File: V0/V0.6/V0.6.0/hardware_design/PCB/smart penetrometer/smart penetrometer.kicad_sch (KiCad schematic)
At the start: 33 parts, among them J1 Screw_Terminal, J2 Conn_01x02, J3 Conn_01x02, J4 Conn_01x07_Female, J5 Conn_02x04, U1 VO615A, U2 ADP7157-3.3, U3 ADS1118IDGS, U4 DS3231M, U5 BME260

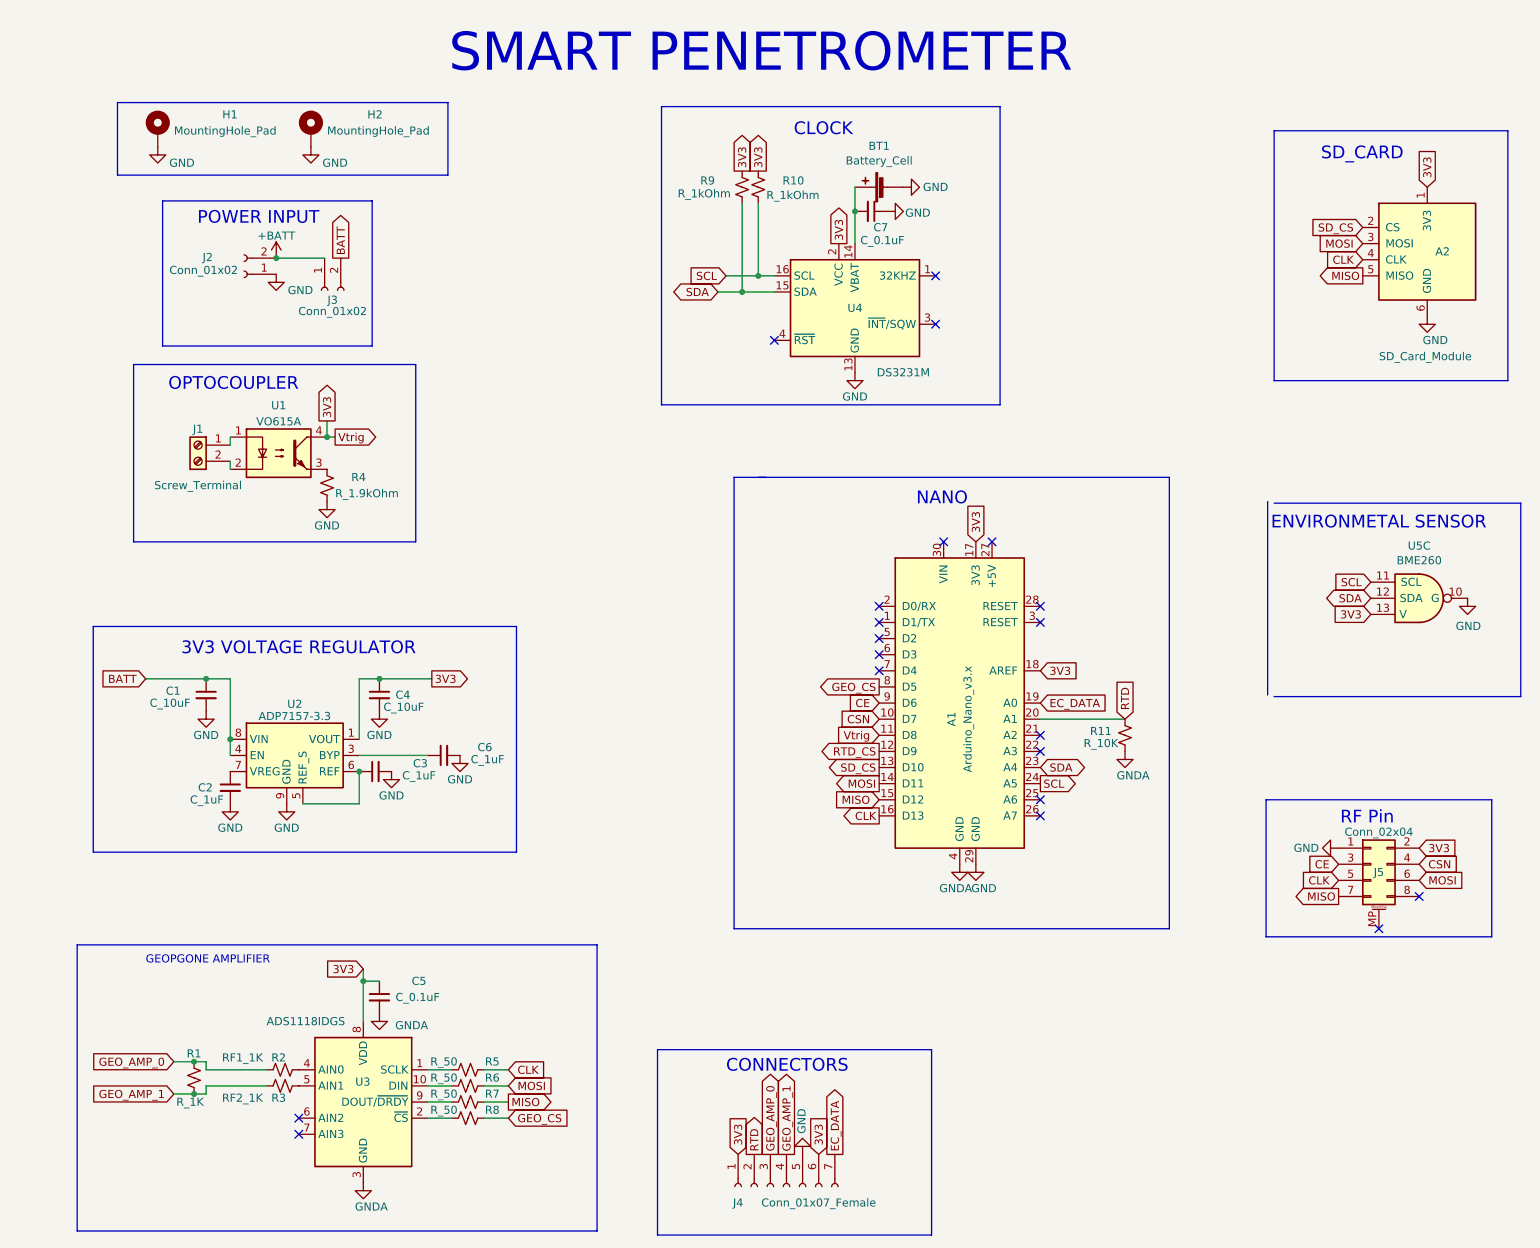
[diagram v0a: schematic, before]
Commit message: correction
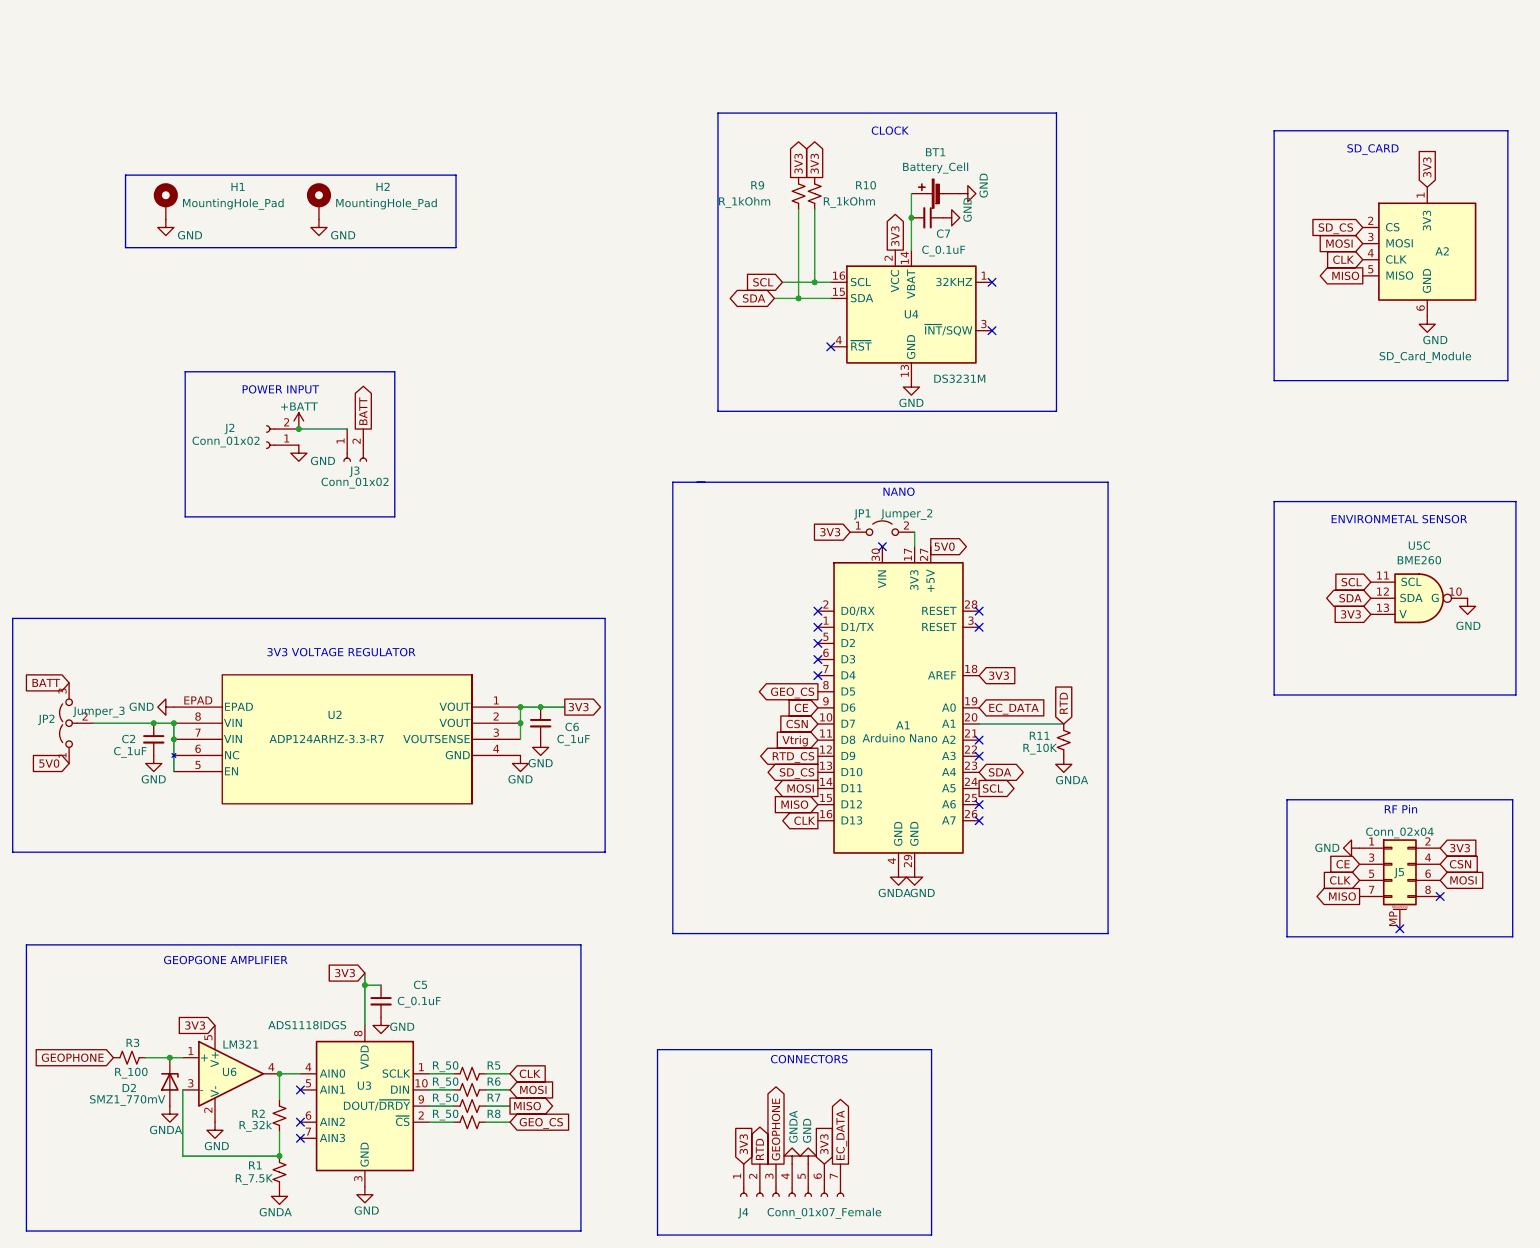
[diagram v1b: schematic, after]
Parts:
- removed C1, C4: C_10uF, Capacitor_SMD:C_1206_3216Metric, symbol Device:C_Small
- removed C3: C_1uF, Capacitor_SMD:C_1206_3216Metric, symbol Device:C_Small
- removed J1: Screw_Terminal, TerminalBlock:TerminalBlock_bornier-2_P5.08mm, symbol Connector:Screw_Terminal_01x02
- removed R4: R_1.9kOhm, Resistor_SMD:R_1206_3216Metric, symbol Device:R_Small_US
- removed U1: VO615A, footprints:Vishay_VOS615A, symbol Isolator:VO615A
- added D2: SMZ1_770mV, Diode_SMD:D_MELF, symbol Diode:SMZxxx
- added JP1: Jumper_2, Connector_PinHeader_2.54mm:PinHeader_1x02_P2.54mm_Vertical, symbol Jumper:Jumper_2_Open
- added JP2: Jumper_3, Connector_PinHeader_2.54mm:PinHeader_1x03_P2.54mm_Vertical, symbol Jumper:Jumper_3_Open
- added U6: LM321, Package_TO_SOT_SMD:SOT-23-5, symbol Amplifier_Operational:LM321
- A1: value Arduino_Nano_v3.x -> Arduino Nano
- R1: value R_1K -> R_7.5K
- R2: value RF1_1K -> R_32k
- R3: value RF2_1K -> R_100
- U2: value ADP7157-3.3 -> ADP124ARHZ-3.3-R7; footprint Package_SO:SOIC-8-1EP_3.9x4.9mm_P1.27mm_EP2.29x3mm -> footprint:RH_8_1_ADI; symbol Regulator_Linear:ADP7142ARDZ-3.3 -> smart penetrometer update-rescue:ADP124ARHZ-3.3-R7
- U5: footprint kitest:TDS_module -> kitest:BME260
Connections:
- net 3V3: now also C6.1, U2.3 (VOUTSENSE), JP1.1 (A), U6.5 (V+); no longer A1.11 (D8), A1.17 (3V3)
- net BATT: now also JP2.3 (B); no longer U2.4 (EN), U2.8 (VIN)
- net GND: now also C5.2, U2.4 (GND), U2.EPAD, U3.3 (GND), U6.2 (V-); no longer U2.9 (GND)
- net GNDA: now also J4.4 (Pin_4), R1.2, D2.2 (A); no longer C5.2, U3.3 (GND)
- net at R2.1, U3.4 (AIN0): now also U6.4
- net at U3.5 (AIN1): no longer R3.1
- net at C2.1, U2.7 (VIN): now also U2.5 (EN), U2.8 (VIN), JP2.2 (C)
- net 5V0: now reaches A1.27 (+5V)
- net 5V0: now also JP2.1 (A)
- net at U2.6 (NC): no longer U2.5 (REF_S)
- net GEO_AMP_0: no longer names the net of R1.1, R2.2
- net GEO_AMP_0: now also U6.3 (-); no longer J4.3 (Pin_3)
- removed net GEO_AMP_1: J4.4 (Pin_4), R1.2, R3.2
- new net: D2.1 (K), R3.2, U6.1 (+)
- new net: A1.17 (3V3), JP1.2 (B)
- new net GEOPHONE: J4.3 (Pin_3), R3.1
- new net Vtrig: A1.11 (D8)
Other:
- note removed: "OPTOCOUPLER"
- note removed: "SMART PENETROMETER"
- moved on the sheet: A1, BT1, C2, C5, C6, C7, H1, H2, J2, J3, J4, J5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
